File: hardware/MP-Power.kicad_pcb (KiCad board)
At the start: 2 copper layers, 17 x 15.7 mm, 12 parts, among them U1 MP1584EN

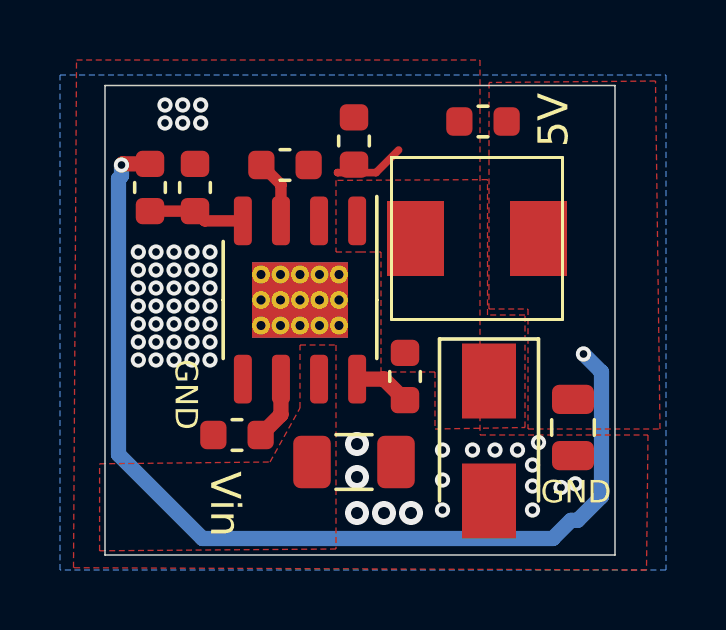
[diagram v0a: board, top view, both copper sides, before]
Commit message: Route one missed trace.
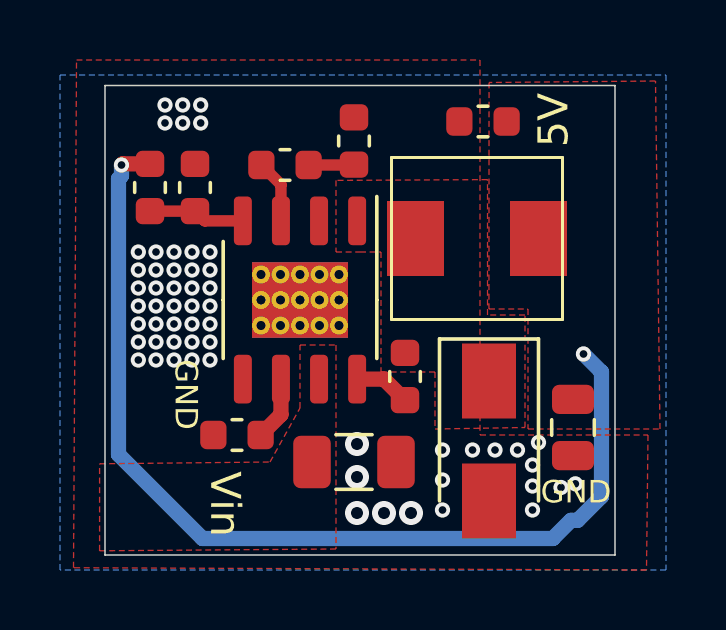
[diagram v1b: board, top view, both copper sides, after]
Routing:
- net GND: track 2.35 -> 0.00 mm
- net Net-(C3-Pad2): track 0.00 -> 1.52 mm
